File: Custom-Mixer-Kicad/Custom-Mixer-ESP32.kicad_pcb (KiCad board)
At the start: 2 copper layers, 192.1 x 118.4 mm, 40 parts, among them J1 Conn_01x08, SW1 RotaryEncoder_Switch, SW10 SW_Push, SW11 SW_Push, SW12 SW_Push, SW13 SW_Push, SW14 SW_Push, SW15 SW_Push, SW16 SW_Push, SW17 SW_Push, SW18 SW_Push, SW19 SW_Push, SW2 RotaryEncoder_Switch, SW21 SW_Push, SW3 SW_Push, SW4 SW_Push, SW5 SW_Push, SW6 SW_Push, SW7 SW_Push, SW8 SW_Push, SW9 SW_Push, U7 ESP32-S3-DevKitC, U8 MCP23017_SP

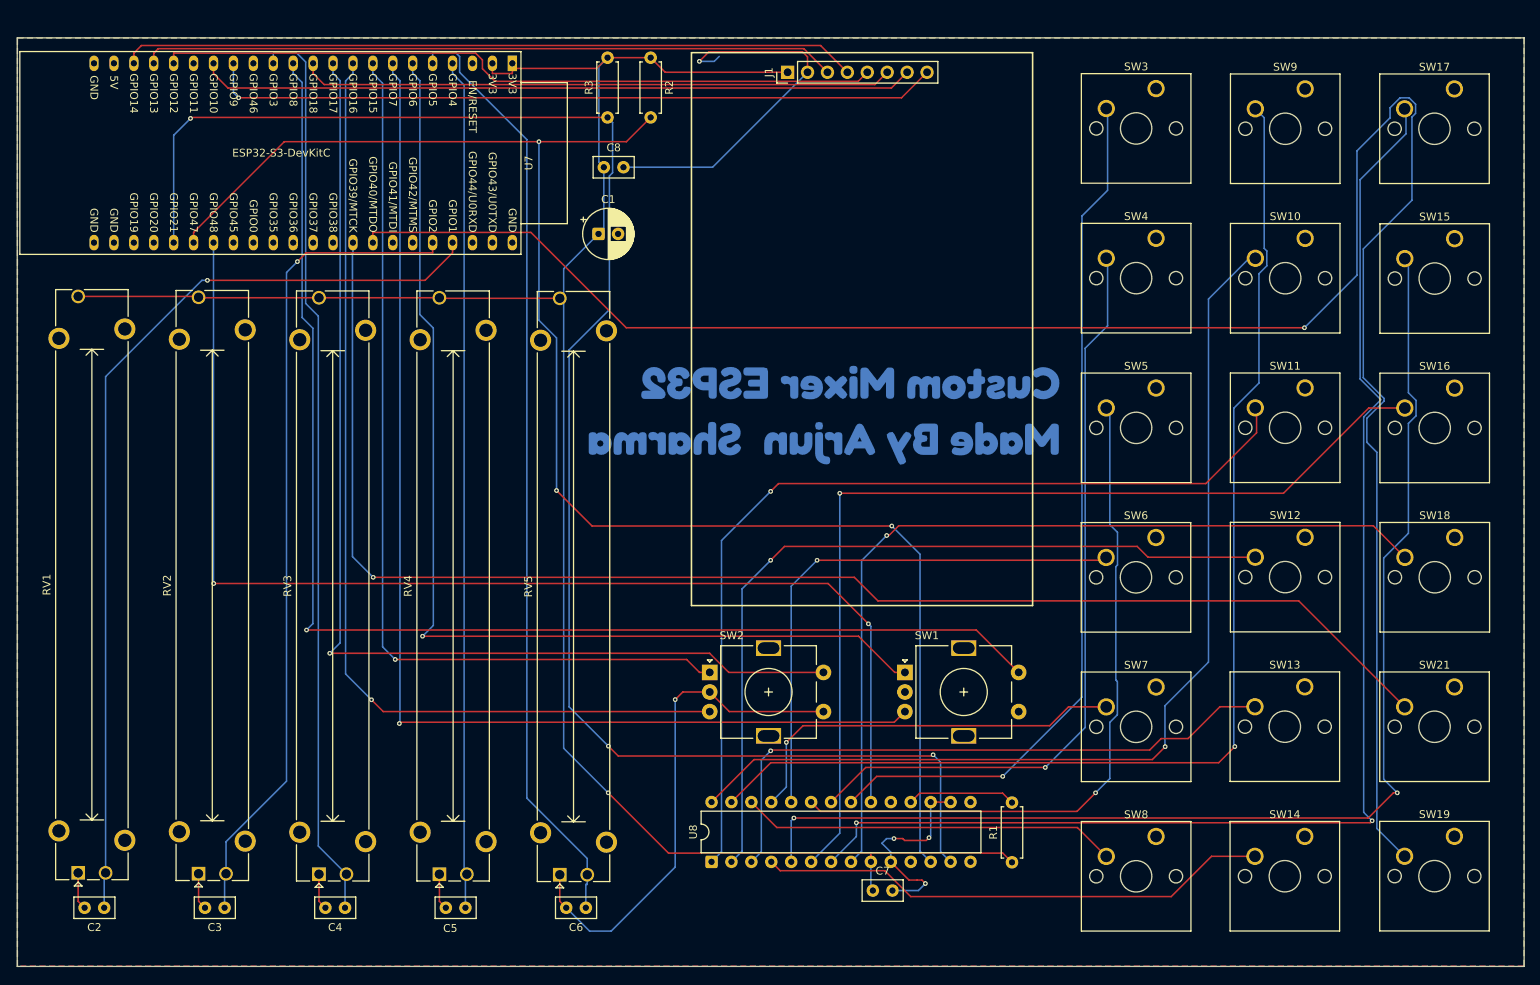
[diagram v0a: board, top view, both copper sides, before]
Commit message: PCB rework completed
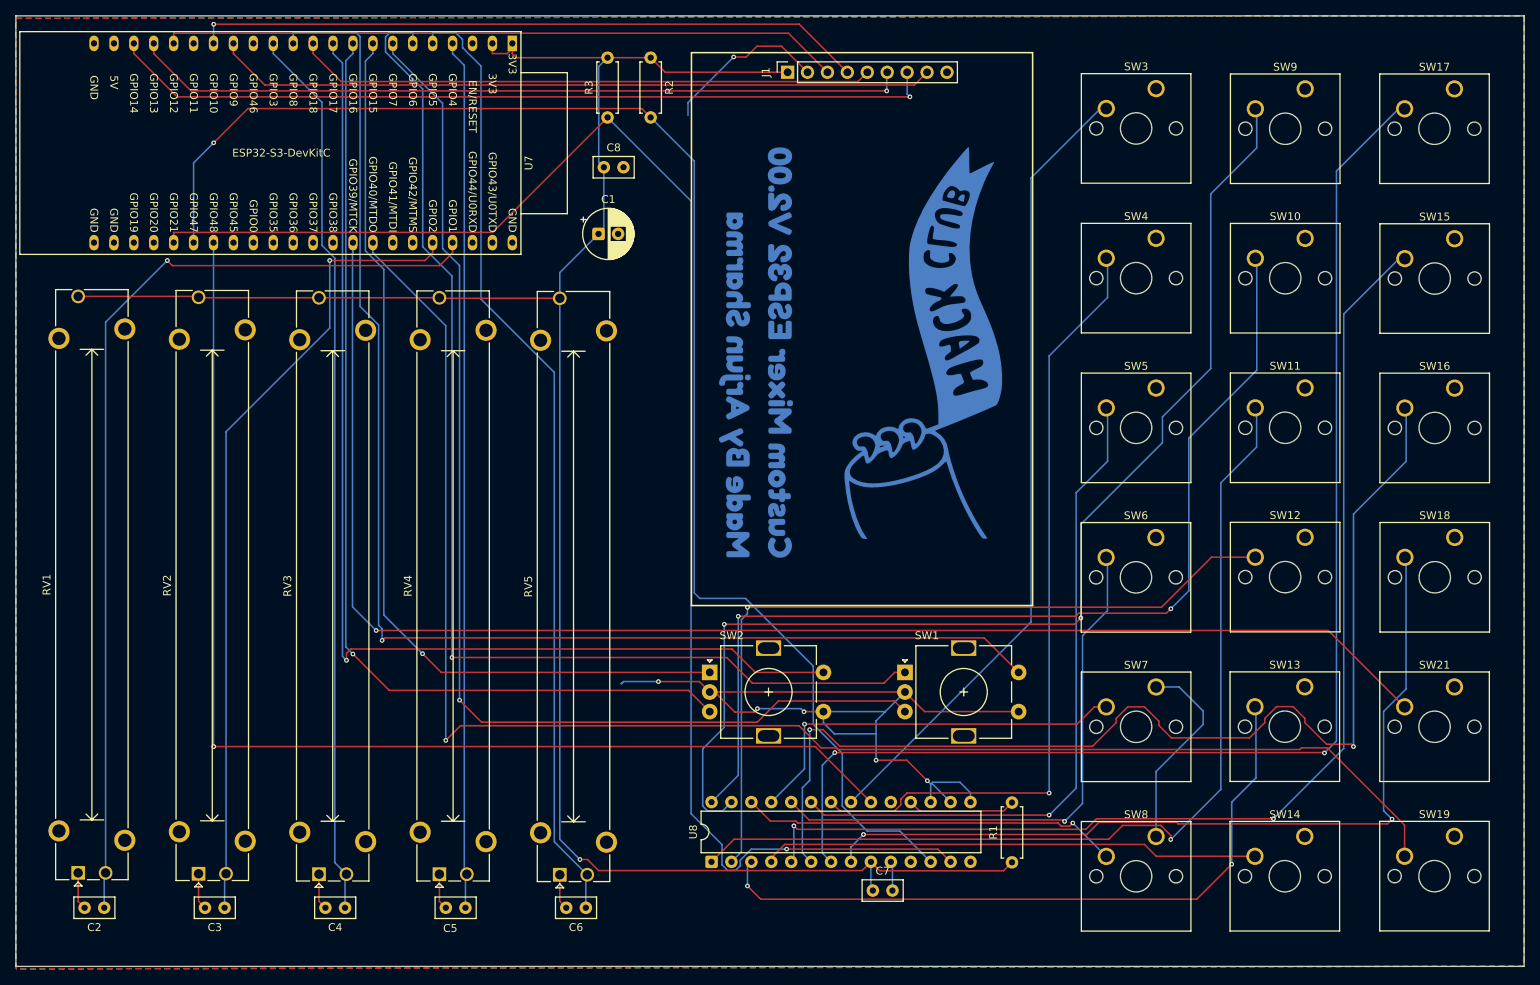
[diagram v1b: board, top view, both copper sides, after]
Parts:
- removed kibuzzard-6987AAB7: G***, kibuzzard-6987AAB7
- added G***: LOGO, Custom-Mixer-Kicad:Hackclublogo, B.Cu at (213.8, 97.8)
- added Goo: LOGO, Custom-Mixer-Kicad:Hackclublogo(fmask), B.Cu at (213.8, 97.8)
- added kibuzzard-698F8E64: G***, kibuzzard-698F8E64, B.Cu at (192.4, 99.1)
- J1: footprint Connector_PinHeader_2.54mm:PinHeader_1x08_P2.54mm_Vertical -> Connector_PinSocket_2.54mm:PinSocket_1x09_P2.54mm_Vertical
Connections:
- J1 pad 3: MOSI -> CS
- J1 pad 4: CLK -> RST
- J1 pad 5: CS -> DC
- J1 pad 6: DC -> MOSI
- J1 pad 7: RST -> CLK
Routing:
- net GPIO 40: track 264.4 -> 199.7 mm
- net GND: track 157.9 -> 190.1 mm, vias 5 -> 6
- net b5: track 125.1 -> 142.7 mm, vias 1 -> 2
- net SDA: track 211.3 -> 195.7 mm, vias 3 -> 1
- net SCL: track 200.6 -> 187.3 mm, vias 3 -> 1
- net CLK: track 94.1 -> 105.8 mm, vias 0 -> 1
- net MOSI: track 88.7 -> 99.1 mm, vias 0 -> 1
- net b2: track 79.3 -> 89.0 mm, vias 1 -> 2
- net b4: track 155.1 -> 145.4 mm
- net GPIO 6: track 138.1 -> 147.3 mm
- net a0: track 111.5 -> 102.3 mm, vias 1 -> 0
- net +3V3: track 262.5 -> 270.2 mm
- net CS: track 92.4 -> 86.7 mm
- net RST: track 91.3 -> 85.8 mm, vias 0 -> 1
- net GPIO 1: track 119.9 -> 124.5 mm
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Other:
- board size 192.1 x 118.4 mm -> 192.3 x 121.2 mm
